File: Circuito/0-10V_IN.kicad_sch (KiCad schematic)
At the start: 6 parts, among them U2 AT3H4B-CUH-S

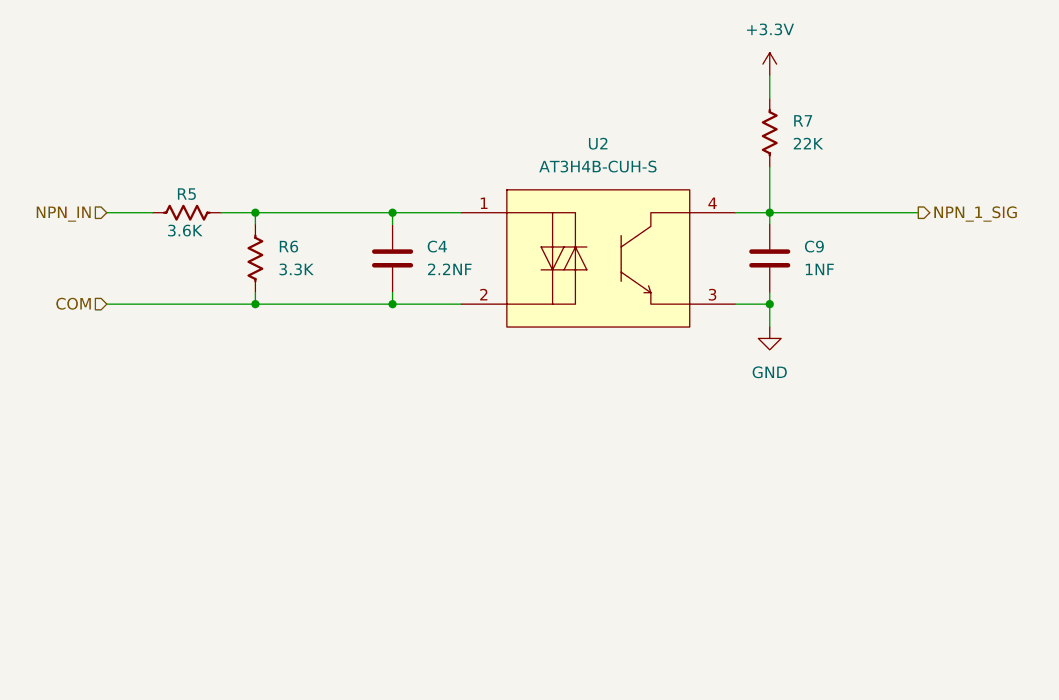
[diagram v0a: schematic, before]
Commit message: commit
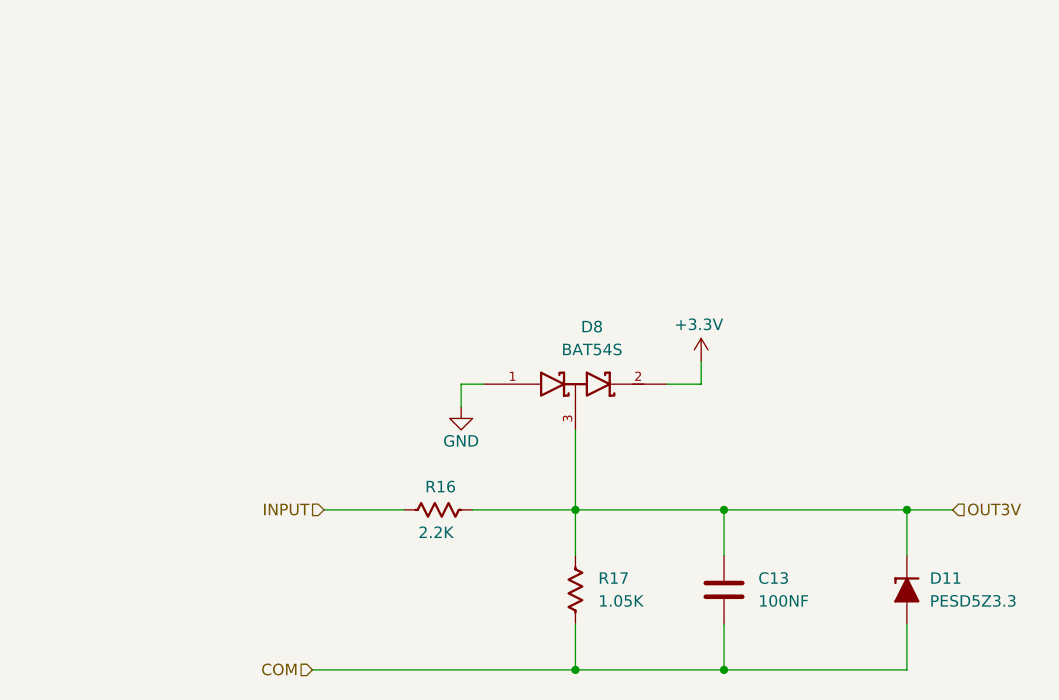
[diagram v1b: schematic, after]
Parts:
- removed C4: 2.2NF, PCM_Capacitor_SMD_AKL:C_0603_1608Metric, symbol Capacitor_AKL:C_0603
- removed C9: 1NF, PCM_Capacitor_SMD_AKL:C_0603_1608Metric, symbol Capacitor_AKL:C_0603
- removed R5: 3.6K, PCM_Resistor_SMD_AKL:R_0603_1608Metric, symbol Resistor_US_AKL:R_0603
- removed R6: 3.3K, PCM_Resistor_SMD_AKL:R_0603_1608Metric, symbol Resistor_US_AKL:R_0603
- removed R7: 22K, PCM_Resistor_SMD_AKL:R_0603_1608Metric, symbol Resistor_US_AKL:R_0603
- removed U2: AT3H4B-CUH-S, easyeda2kicad:SSOP-4_L2.7-W4.6-P1.27-LS7.0-TL, symbol easyeda2kicad:AT3H4B-CUH-S
- added C13: 100NF, PCM_Capacitor_SMD_AKL:C_0603_1608Metric, symbol Capacitor_AKL:C_0603
- added D11: PESD5Z3.3, PCM_Diode_SMD_AKL:D_SOD-523, symbol Diode_TVS_AKL:PESD5Z3.3
- added D8: BAT54S, PCM_4ms_Package_SOT:SOT23-3_PO132, symbol 4ms_Diode:BAT54S
- added R16: 2.2K, PCM_Resistor_SMD_AKL:R_0603_1608Metric, symbol Resistor_US_AKL:R_0603
- added R17: 1.05K, PCM_Resistor_SMD_AKL:R_0603_1608Metric, symbol Resistor_US_AKL:R_0603
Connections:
- net +3.3V: now also D8.2 (cathode)
- net COM: now also C13.2, D11.2 (A), R17.2
- net GND: now also D8.1 (Anode)
- new net INPUT: R16.1
- new net OUT3V: C13.1, D11.1 (K), D8.3 (AK), R16.2, R17.1
